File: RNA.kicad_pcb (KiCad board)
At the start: 2 copper layers, 126 x 85 mm, 86 parts, among them J1 USB_B_Micro, J2 AudioJack4, J3 Conn_01x06, SW1 SW_Push, SW11 SW_Push_45deg, SW12 SW_Push_45deg, SW13 SW_Push_45deg, SW14 SW_Push_45deg, SW15 SW_Push_45deg, SW16 SW_Push_45deg, SW2 SW_Push, SW21 SW_Push_45deg, SW22 SW_Push_45deg, SW23 SW_Push_45deg, SW24 SW_Push_45deg, SW25 SW_Push_45deg, SW26 SW_Push_45deg, SW31 SW_Push_45deg, SW32 SW_Push_45deg, SW33 SW_Push_45deg, SW34 SW_Push_45deg, SW35 SW_Push_45deg, SW36 SW_Push_45deg, SW41 SW_Push_45deg, SW42 SW_Push_45deg, SW43 SW_Push_45deg, SW44 SW_Push_45deg, SW45 SW_Push_45deg, SW46 SW_Push_45deg, SW47 SW_Push_45deg, SW51 SW_Push_45deg, SW52 SW_Push_45deg, SW53 SW_Push_45deg, SW54 SW_Push_45deg, SW55 SW_Push_45deg, SW56 SW_Push_45deg, SW57 SW_Push_45deg, U1 STM32F072C8Tx, U2 USBLC6-2SC6, U3 MIC5219-3.3YM5

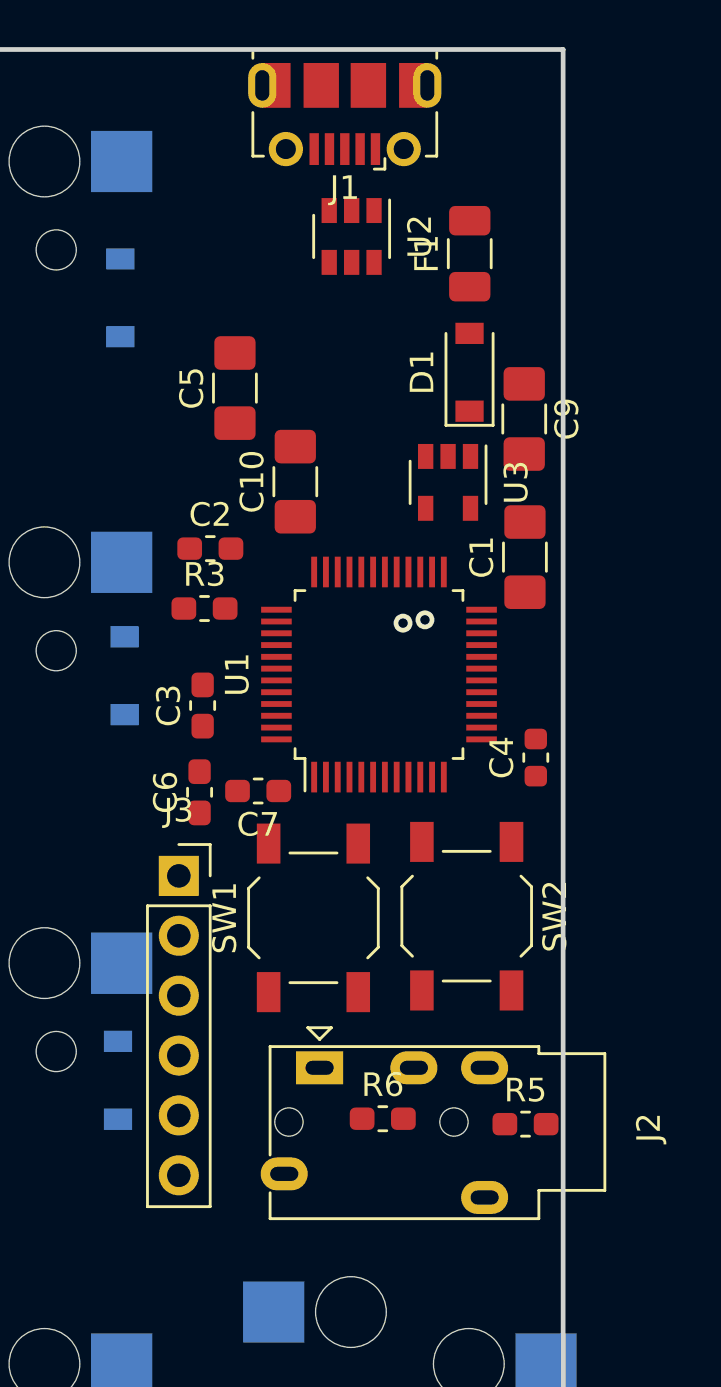
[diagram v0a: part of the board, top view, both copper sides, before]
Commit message: wip"
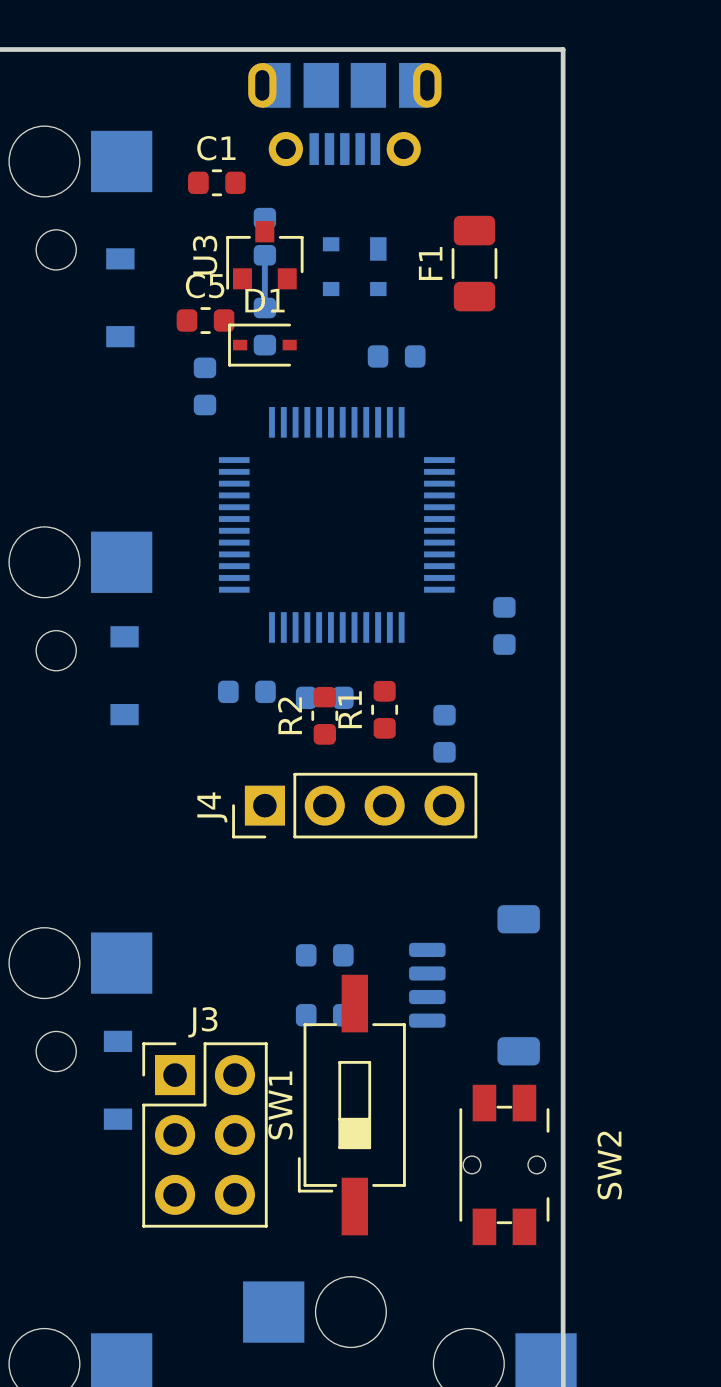
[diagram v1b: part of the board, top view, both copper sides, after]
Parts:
- removed C10, C9: 10u, Capacitor_SMD:C_1206_3216Metric_Pad1.42x1.75mm_HandSolder
- added J4: AudioJack4, Connector_PinHeader_2.54mm:PinHeader_1x04_P2.54mm_Vertical, F.Cu at (133.3, 52.1)
- added R1: R_Small, Resistor_SMD:R_0603_1608Metric, F.Cu at (138.4, 48.0)
- added R2: R_Small, Resistor_SMD:R_0603_1608Metric, F.Cu at (135.9, 48.3)
- added R4: 39k, Resistor_SMD:R_0603_1608Metric, B.Cu at (133.3, 27.9)
- added R7: 68k, Resistor_SMD:R_0603_1608Metric, B.Cu at (133.3, 31.8)
- C1: value 4.7u -> 1u; footprint Capacitor_SMD:C_1206_3216Metric_Pad1.42x1.75mm_HandSolder -> Capacitor_SMD:C_0603_1608Metric
- C2, C3: value 1n -> 100n; footprint Capacitor_SMD:C_0603_1608Metric_Pad1.05x0.95mm_HandSolder -> Capacitor_SMD:C_0603_1608Metric; moved to B.Cu
- C4, J1, U1: moved to B.Cu
- C5: footprint Capacitor_SMD:C_1206_3216Metric_Pad1.42x1.75mm_HandSolder -> Capacitor_SMD:C_0603_1608Metric
- C6, C7: footprint Capacitor_SMD:C_0603_1608Metric_Pad1.05x0.95mm_HandSolder -> Capacitor_SMD:C_0603_1608Metric; moved to B.Cu
- D1: value D_Small -> D_Schottky_Small; footprint Diode_SMD:D_SOD-123 -> Diode_SMD:D_SOD-323
- J2: footprint Connector_Audio:Jack_3.5mm_PJ320E_Horizontal -> Connector_JST:JST_SH_SM04B-SRSS-TB_1x04-1MP_P1.00mm_Horizontal; moved to B.Cu
- J3: footprint Connector_PinSocket_2.54mm:PinSocket_1x06_P2.54mm_Vertical -> Connector_PinHeader_2.54mm:PinHeader_2x03_P2.54mm_Vertical
- R3, R5, R6: footprint Resistor_SMD:R_0603_1608Metric_Pad1.05x0.95mm_HandSolder -> Resistor_SMD:R_0603_1608Metric; moved to B.Cu
- SW1: value SW_Push -> SW_SPST; footprint Button_Switch_SMD:SW_SPST_TL3342 -> Button_Switch_SMD:SW_DIP_SPSTx01_Slide_6.7x4.1mm_W8.61mm_P2.54mm_LowProfile
- SW2: footprint Button_Switch_SMD:SW_SPST_TL3342 -> Button_Switch_SMD:Panasonic_EVQPUL_EVQPUC
- U2: value USBLC6-2SC6 -> PRTR5V0U2X; footprint Package_TO_SOT_SMD:SOT-23-6 -> random-keyboard-parts:SOT143B; moved to B.Cu
- U3: value MIC5219-3.3YM5 -> MCP1703A-3302_SOT23; footprint Package_TO_SOT_SMD:SOT-23-5 -> Package_TO_SOT_SMD:SOT-23
- moved C1 20.6 mm to (131.3, 25.7), turned to 0 degrees
- moved C6 17.2 mm to (130.8, 34.3), turned to 270 degrees
- moved C3 16.9 mm to (138.9, 33.0), turned to 0 degrees
- moved C2 12.9 mm to (143.5, 44.5), turned to 90 degrees
- moved C4 12.6 mm to (132.6, 47.2), turned to 0 degrees
- moved U3 12.4 mm to (133.3, 28.7), turned to 90 degrees
- moved R3 11.5 mm to (141.0, 49.0), turned to 90 degrees
- moved SW2 10.7 mm to (143.5, 67.3)
- moved R5 9.69 mm to (135.9, 61.0)
- moved D1 8.76 mm to (133.3, 32.5), turned to 0 degrees
- moved J3 8.45 mm to (129.5, 63.5)
- moved SW1 8.13 mm to (137.2, 64.8)
- moved J2 7.44 mm to (142.2, 59.7)
- moved R6 7.35 mm to (135.9, 58.4), turned to 180 degrees
- moved U1 6.59 mm to (136.4, 40.2)
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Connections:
- net Net-(U1-Pad39) renamed SWO
- C1 pad 1: VDD -> Net-(C1-Pad1)
- D1 pad 1: Net-(C9-Pad1) -> Net-(C1-Pad1)
- J1 pad 2: Net-(J1-Pad2) -> D-
- J1 pad 3: Net-(J1-Pad3) -> D+
- R5 pad 2: Net-(J2-PadR2) -> Net-(J2-Pad3)
- R6 pad 2: Net-(J2-PadR1) -> Net-(J2-Pad2)
- U1 pad 38: Net-(U1-Pad38) -> VBUS_SENSE
- U1 pad 44: BOOT0 -> Net-(U1-Pad44)
- U1 pad 5: Net-(U1-Pad5) -> BOOT0
- U2 pad 1: Net-(J1-Pad2) -> GND
- U2 pad 2: GND -> D+
- U2 pad 3: Net-(J1-Pad3) -> D-
- U2 pad 4: D+ -> VBUS
- U3 pad 1: Net-(C9-Pad1) -> GND
- U3 pad 2: GND -> VDD
- U3 pad 3: Net-(C9-Pad1) -> Net-(C1-Pad1)
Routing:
- net VBUS_SENSE: track 0.00 -> 2.23 mm
- net (no net): vias 2 -> 0
